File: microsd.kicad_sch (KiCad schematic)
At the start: 8 parts, among them J7 503398-1892

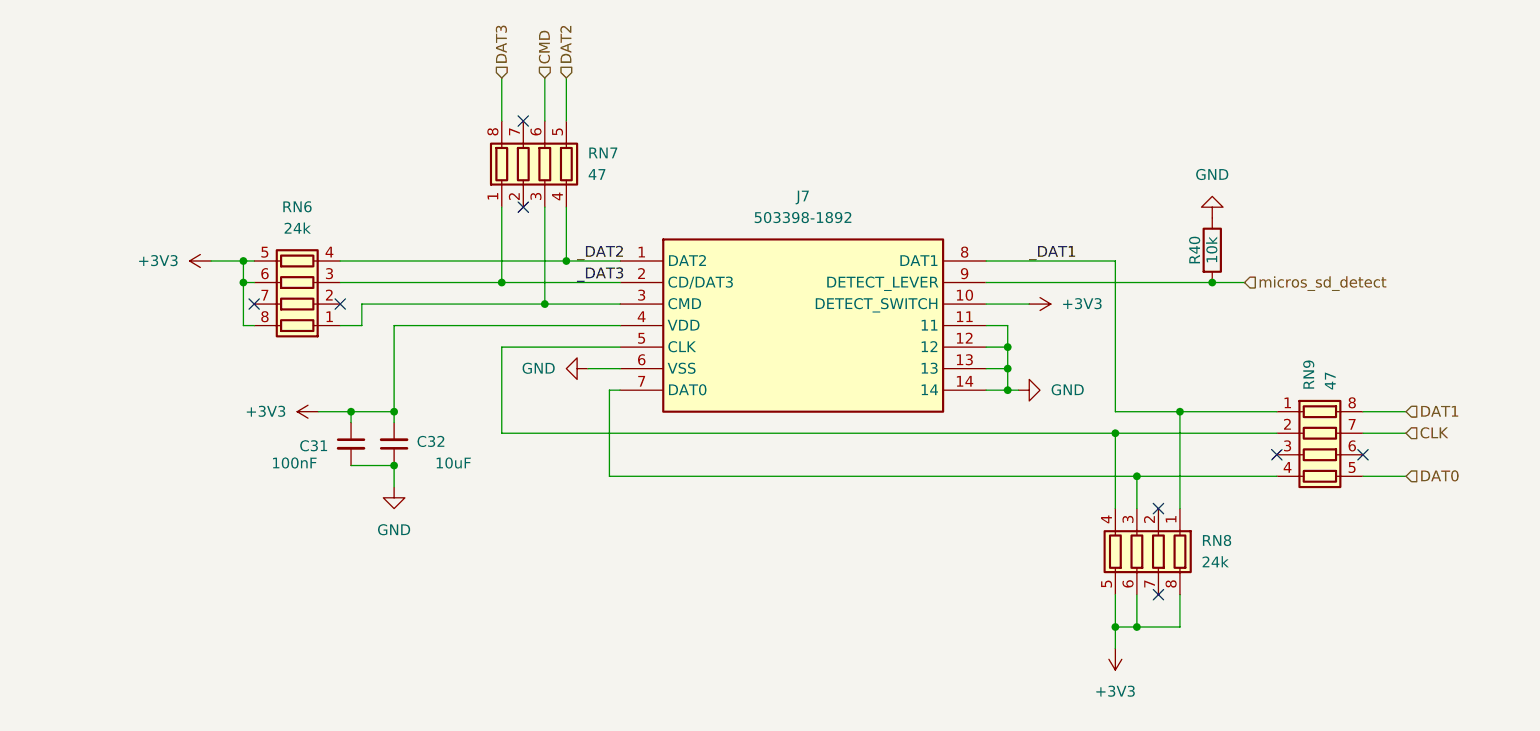
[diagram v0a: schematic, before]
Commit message: Tentativo di Sbroglio
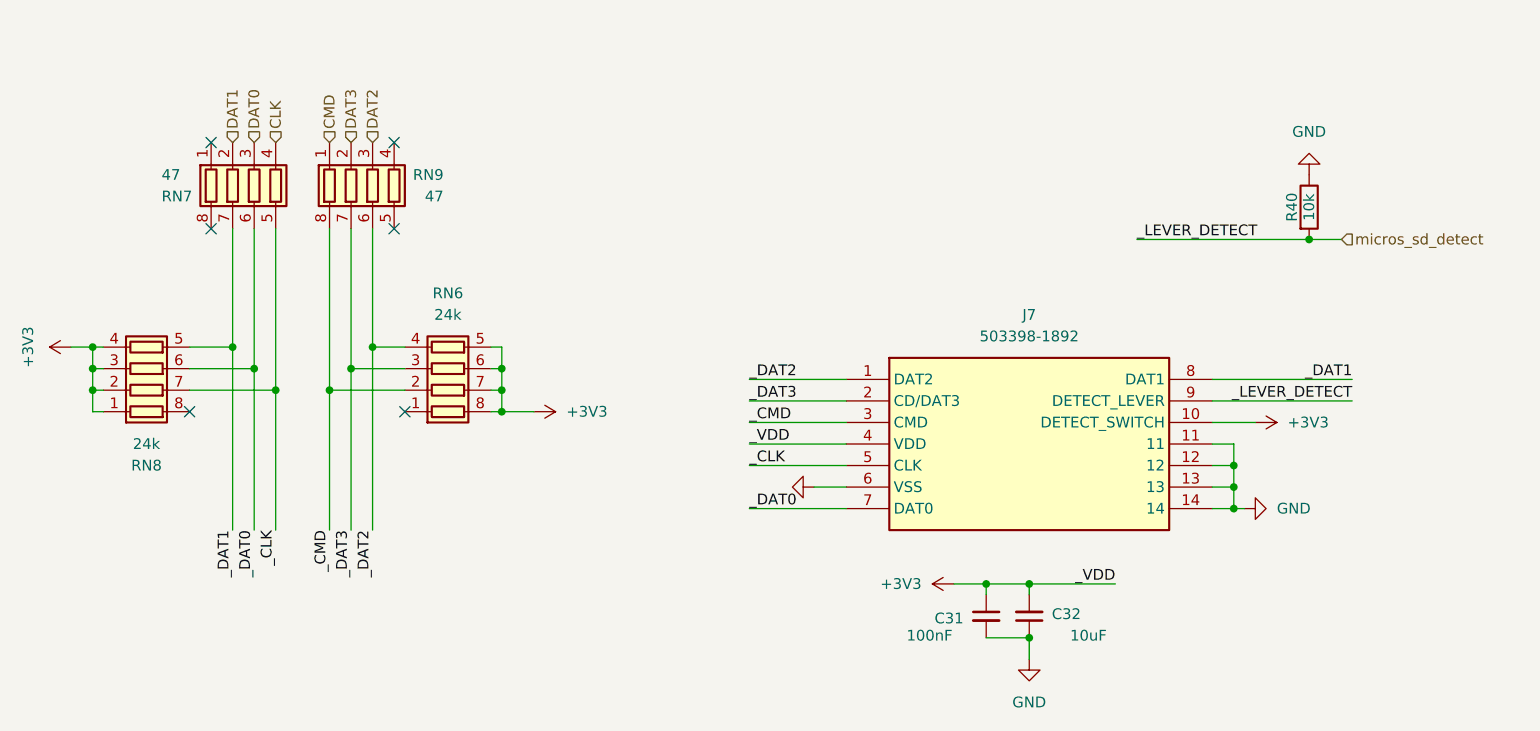
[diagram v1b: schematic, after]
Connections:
- net +3V3: now also RN6.7 (R2.2), RN8.1 (R1.1), RN8.2 (R2.1), RN8.3 (R3.1), RN8.4 (R4.1); no longer RN8.5 (R4.2), RN8.6 (R3.2), RN8.8 (R1.2)
- net CLK: now also RN7.4 (R4.1); no longer RN9.7 (R2.2)
- net CMD: now also RN9.1 (R1.1); no longer RN7.6 (R3.2)
- net DAT0: now also RN7.3 (R3.1); no longer RN9.5 (R4.2)
- net DAT1: now also RN7.2 (R2.1); no longer RN9.8 (R1.2)
- net DAT2: now also RN9.3 (R3.1); no longer RN7.5 (R4.2)
- net DAT3: now also RN9.2 (R2.1); no longer RN7.8 (R1.2)
- net _DAT1: now also RN7.7 (R2.2), RN8.5 (R4.2); no longer RN8.1 (R1.1), RN9.1 (R1.1)
- net _DAT2: now also RN9.6 (R3.2); no longer RN7.4 (R4.1)
- net _DAT3: now also RN9.7 (R2.2); no longer RN7.1 (R1.1)
- net _CLK: now reaches RN8.7 (R2.2)
- net _CLK: now also J7.5 (CLK), RN7.5 (R4.2)
- net _CMD: now reaches RN6.2 (R2.1)
- net _CMD: now also J7.3 (CMD), RN9.8 (R1.2)
- new net _DAT0: J7.7 (DAT0), RN7.6 (R3.2), RN8.6 (R3.2)
- now unconnected: RN6.1 (R1.1), RN9.4 (R4.1)
- no-connect marks 8 -> 6
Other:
- moved on the sheet: C31, C32, J7, R40, RN6, RN7, RN8, RN9
